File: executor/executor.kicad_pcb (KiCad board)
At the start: 4 copper layers, 58 x 58 mm, 135 parts, among them J1 XT30PW(2+2), Q1 WNM6006, Q2 WNM6006, Q3 WNM6006, Q4 WNM6006, Q5 WNM6006, Q6 WNM6006, U1 WD1601E, U2 DRV8323SRTAT, U3 GD32F303RETx, U4 TCAN4550RGYRQ1, U5 AS5047P-ATSM, U6 QMA7981, Y1 8M, Y2 40M

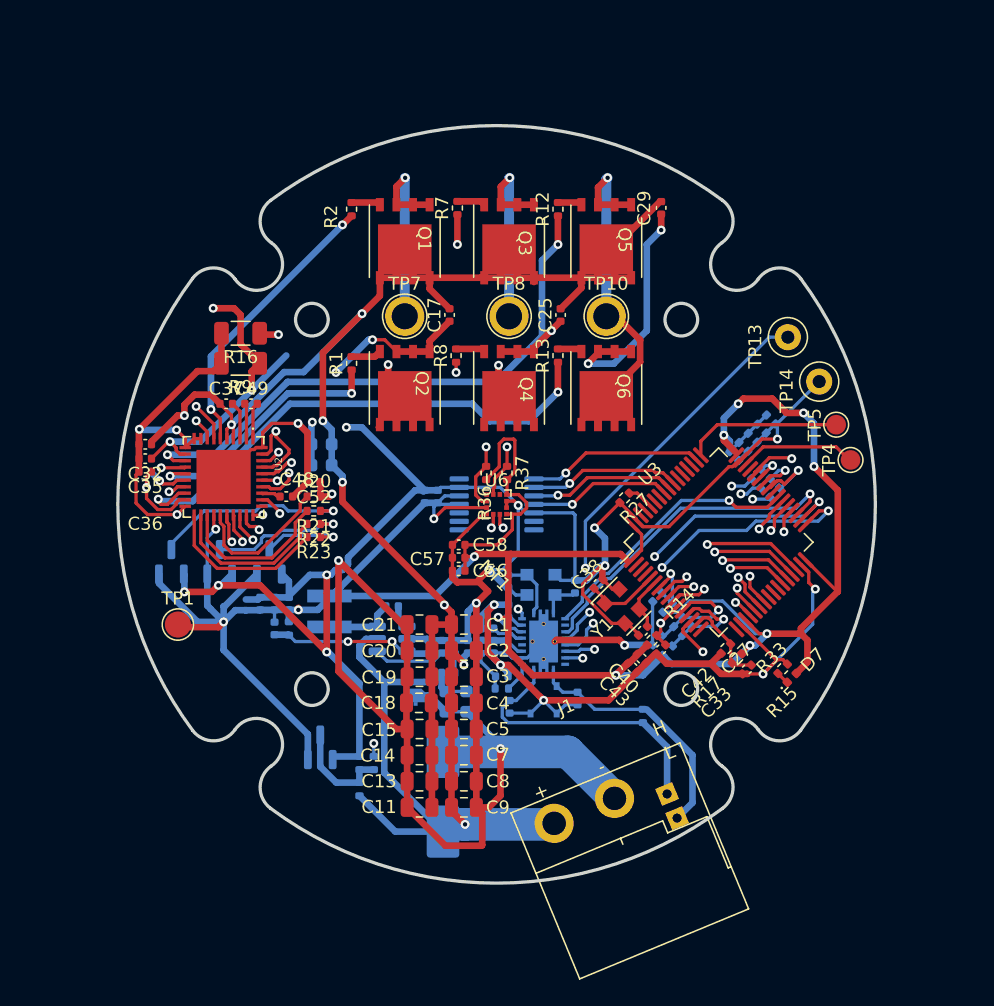
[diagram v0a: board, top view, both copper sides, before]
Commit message: [New] Complete executor ver 0.1
Signed-off-by: Homalozoa <nx.tardis@gmail.com>
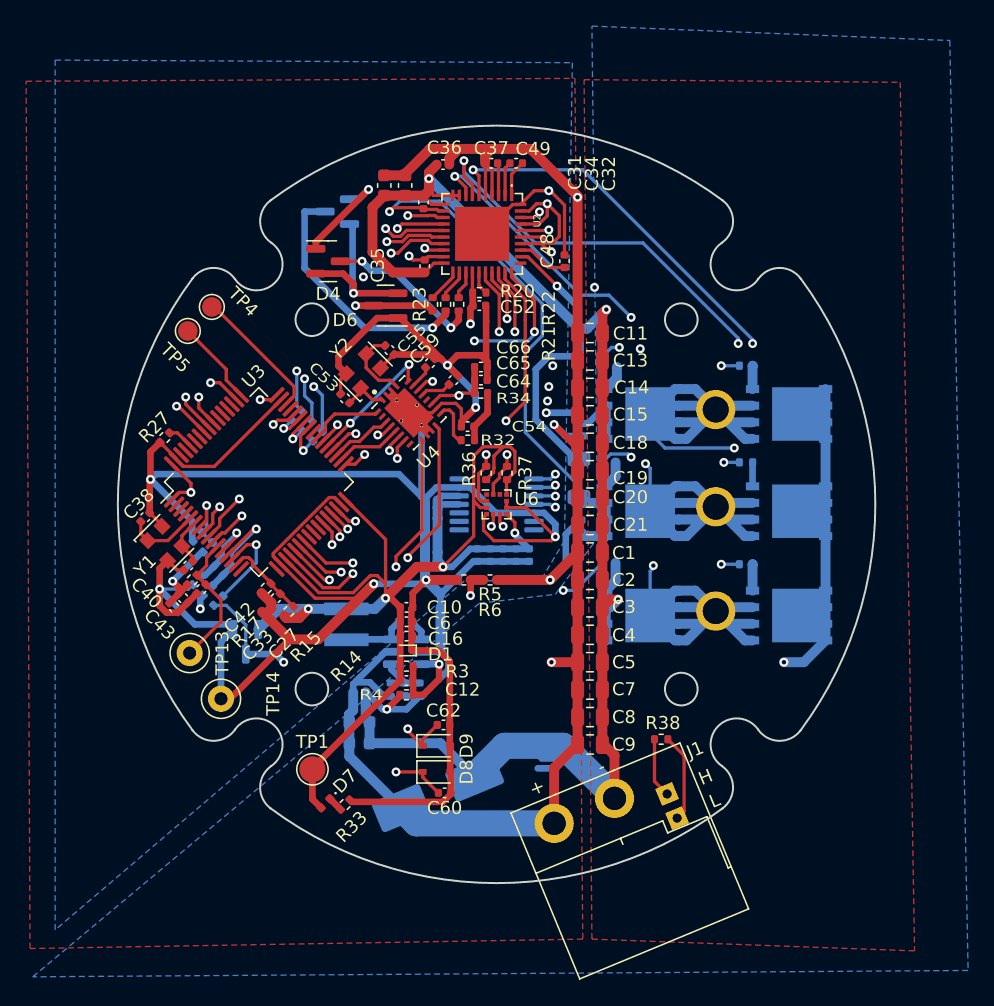
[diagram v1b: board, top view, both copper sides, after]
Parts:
- removed R16: 0.001R, Resistor_SMD:R_1206_3216Metric
- C10, C12, C16, C31, C34, C53, C54, C55, C59, C6, C60, C62, C64, C65, C66, D1, D4, D6, D8, D9, R3, R32, R34, R38, R4, R5, R6, U4, Y2: moved to F.Cu
- C17, C25, C29, C56, C57, C58, NT1, Q1, Q2, Q3, Q4, Q5, Q6, R1, R12, R13, R2, R7, R8, R9, TP10, TP7, TP8: moved to B.Cu
- moved TP14 51.8 mm to (53.9, 74.9)
- moved TP13 51.8 mm to (51.5, 71.4)
- moved TP4 50.3 mm to (53.2, 44.9), turned to 135 degrees
- moved TP5 50.2 mm to (51.4, 46.7), turned to 135 degrees
- moved Q1 41.1 mm to (97.5, 68.3), turned to 0 degrees
- moved R2 40.6 mm to (94.1, 64.6), turned to 0 degrees
- moved C11 38.6 mm to (82.2, 46.9), turned to 0 degrees
- moved D7 37.0 mm to (61.9, 82.9), turned to -135 degrees
- moved C27 36.5 mm to (58.1, 67.2)
- moved C45 35.5 mm to (53.7, 65.1)
- moved R17 35.5 mm to (51.7, 65.8)
- moved U3 35.5 mm to (56.8, 58.3)
- moved C33 35.5 mm to (52.4, 66.5)
- moved C39 35.5 mm to (52.1, 62.5)
- moved C46 35.5 mm to (54.4, 64.4)
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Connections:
- net IAN renamed GNDA
- net VM renamed +24V
- R29 pad 2: PWM_C -> PWM_B
- R30 pad 2: PWM_B -> PWM_C
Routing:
- net GND: track 240.9 -> 285.5 mm, vias 17 -> 10
- net CAN_L: track 19.1 -> 60.2 mm, vias 0 -> 2
- net A: track 44.5 -> 85.2 mm
- net ECD_MOSI: track 10.9 -> 47.5 mm, vias 1 -> 2
- net ECD_MISO: track 11.2 -> 44.6 mm, vias 1 -> 2
- net CAN_H: track 22.1 -> 54.7 mm, vias 0 -> 2
- net ICP: track 69.6 -> 37.8 mm, vias 4 -> 3
- net ECD_SCK: track 11.6 -> 41.2 mm, vias 1 -> 2
- net +24V: track 170.9 -> 200.2 mm, vias 8 -> 6
- net Net-(R31-Pad1): track 36.3 -> 7.32 mm, vias 2 -> 1
- net TCAN_SDO: track 33.0 -> 5.13 mm, vias 3 -> 0
- net TEMP_MOTOR: track 38.3 -> 10.6 mm, vias 2 -> 0
- net VGL_A: track 19.6 -> 46.4 mm
- net TCAN_SDI: track 31.8 -> 5.01 mm, vias 3 -> 2
- net VGH_A: track 21.8 -> 48.5 mm, vias 2 -> 3
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- added copper zone on In2.Cu, net +24V
- added copper zone on In1.Cu, net +3V3
- added copper zone on B.Cu, net GND
- added copper zone on F.Cu, net GND
- added copper zone on B.Cu, net GNDA
- added copper zone on F.Cu, net GNDA
